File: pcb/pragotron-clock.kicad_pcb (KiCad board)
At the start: 2 copper layers, 60 x 60 mm, 11 parts, among them J1 Conn_01x02, J2 Conn_01x03, J3 Conn_01x03, J4 Conn_01x02, U1 L293D, U2 ESP32_DEVCITV1

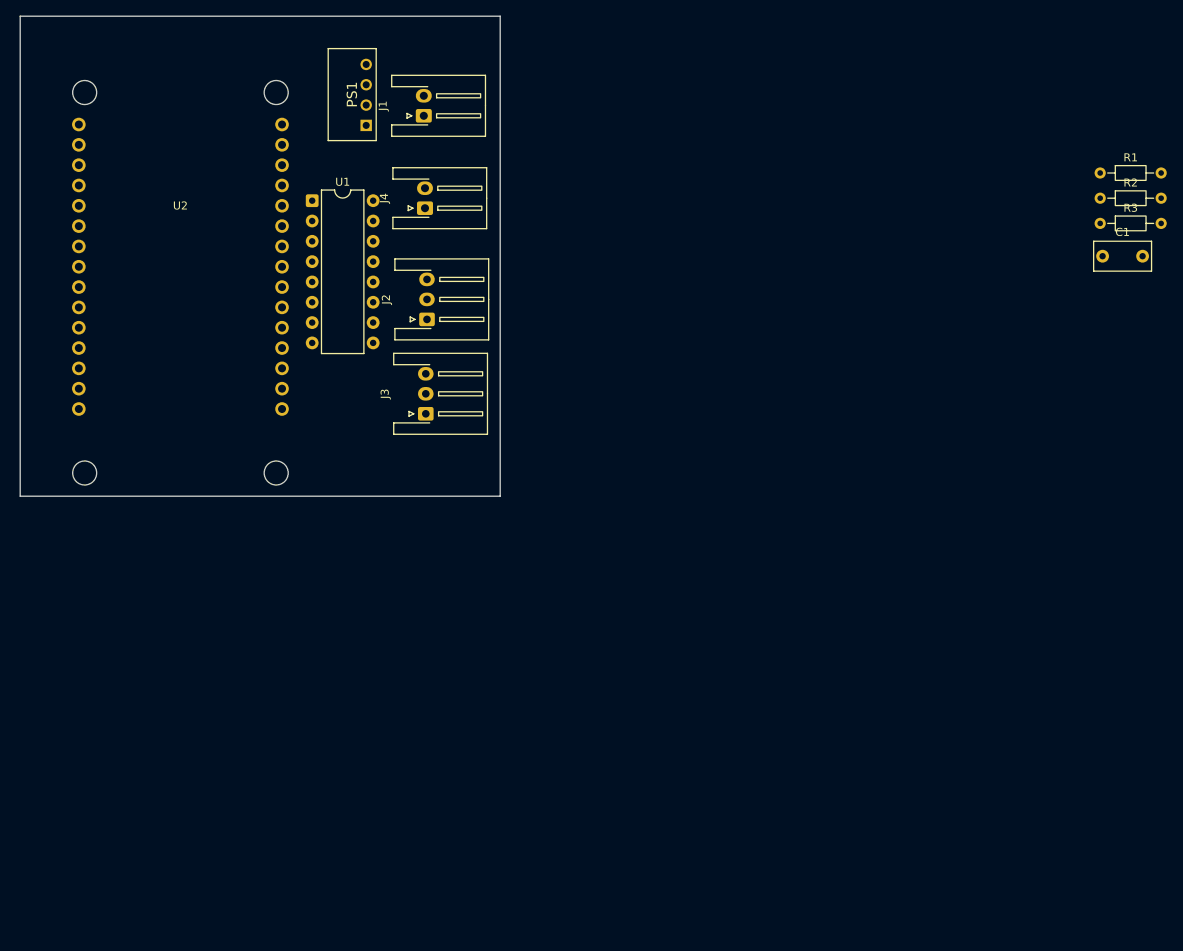
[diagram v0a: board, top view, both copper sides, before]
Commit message: schematic
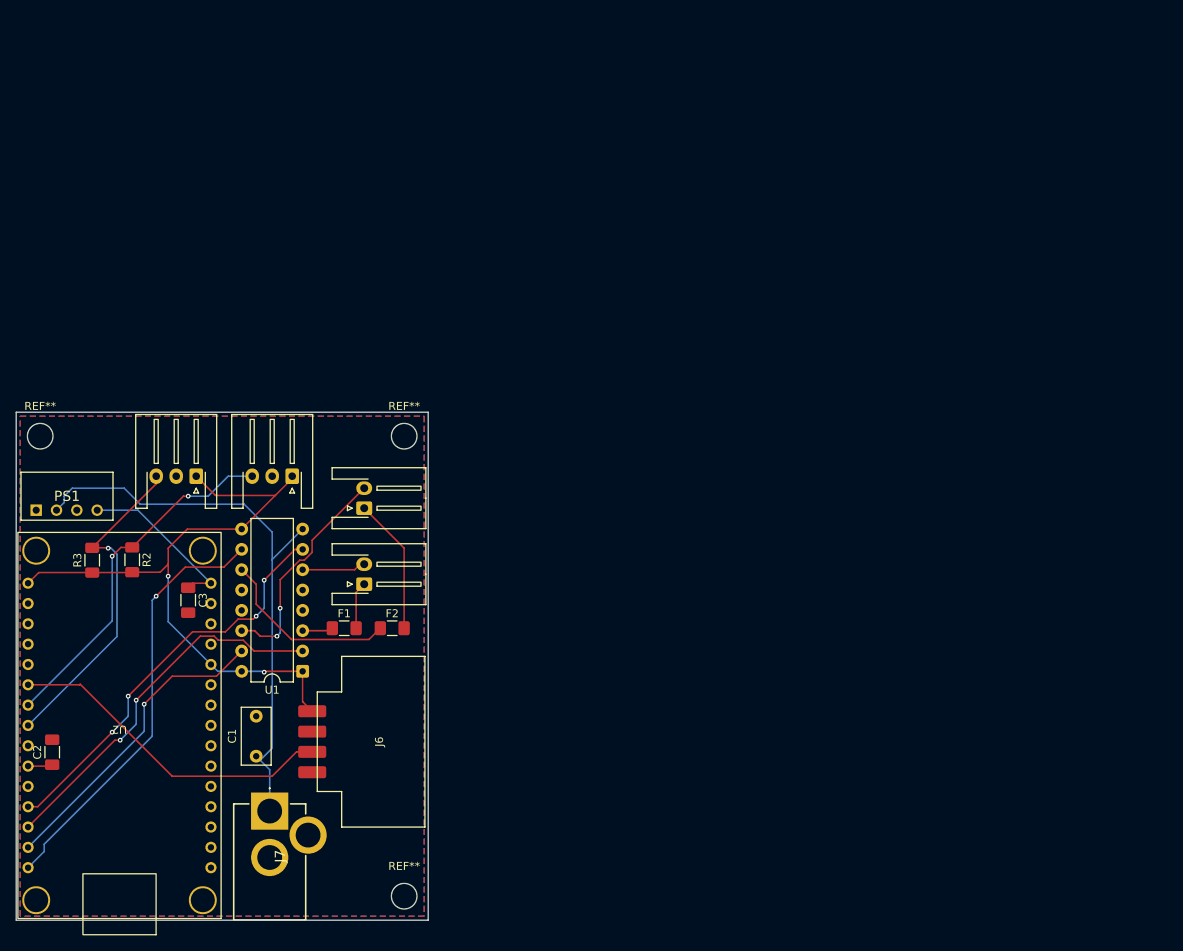
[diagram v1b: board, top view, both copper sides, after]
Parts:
- removed J4: Conn_01x02, Connector_JST:JST_XH_S2B-XH-A-1_1x02_P2.50mm_Horizontal
- removed R1: 47K, Resistor_THT:R_Axial_DIN0204_L3.6mm_D1.6mm_P7.62mm_Horizontal
- added C2: 100n, Capacitor_SMD:C_1206_3216Metric_Pad1.33x1.80mm_HandSolder, F.Cu at (84.0, 142.0)
- added C3: 100n, Capacitor_SMD:C_1206_3216Metric_Pad1.33x1.80mm_HandSolder, F.Cu at (101.0, 123.0)
- added F1: Fuse, Fuse:Fuse_1206_3216Metric_Pad1.42x1.75mm_HandSolder, F.Cu at (120.5, 126.5)
- added F2: Fuse, Fuse:Fuse_1206_3216Metric_Pad1.42x1.75mm_HandSolder, F.Cu at (126.5, 126.5)
- added J5: Conn_01x02, Connector_JST:JST_XH_S2B-XH-A-1_1x02_P2.50mm_Horizontal, F.Cu at (123.0, 111.5)
- added J6: Conn_01x04, JS_Local:DCF77, F.Cu at (125.4, 140.7)
- added J7: 694108301002, JS_Local:694108301002, F.Cu at (111.2, 149.4)
- added REF**: MountingHole_3.2mm_M3_DIN965, MountingHole:MountingHole_3.2mm_M3_DIN965, F.Cu at (128.0, 160.0)
- added REF**: MountingHole_3.2mm_M3_DIN965, MountingHole:MountingHole_3.2mm_M3_DIN965, F.Cu at (128.0, 102.5)
- added REF**: MountingHole_3.2mm_M3_DIN965, MountingHole:MountingHole_3.2mm_M3_DIN965, F.Cu at (82.5, 102.5)
- R2, R3: footprint Resistor_THT:R_Axial_DIN0204_L3.6mm_D1.6mm_P7.62mm_Horizontal -> Resistor_SMD:R_1206_3216Metric_Pad1.30x1.75mm_HandSolder
- U2: value ESP32_DEVCITV1 -> ~; footprint JS_Local:ESP32_DEVKITV1 -> JS_Local:ESP8266_12E_DEVKIT
- moved R3 132.8 mm to (89.0, 118.0), turned to 90 degrees
- moved R2 129.2 mm to (94.0, 118.0), turned to -90 degrees
- moved C1 122.9 mm to (109.5, 142.5), turned to 90 degrees
- moved U2 75.3 mm to (92.4, 138.7), turned to 180 degrees
- moved PS1 63.4 mm to (82.0, 111.8), turned to 0 degrees
- moved J1 59.0 mm to (123.0, 121.0)
- moved U1 58.8 mm to (115.3, 131.9), turned to 180 degrees
- moved J3 29.7 mm to (102.0, 107.5), turned to 180 degrees
- moved J2 25.8 mm to (114.0, 107.5), turned to 180 degrees
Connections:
- J2 pad 1: Net-(J2-Pin_1) -> +3V3
- J2 pad 3: Net-(J2-Pin_3) -> /SENS2
- J3 pad 1: Net-(J2-Pin_1) -> +3V3
- J3 pad 3: Net-(J3-Pin_3) -> /SENS1
- R2 pad 1: Net-(J2-Pin_3) -> /SENS2
- R2 pad 2: Net-(J2-Pin_1) -> +3V3
- R3 pad 1: Net-(J2-Pin_1) -> +3V3
- R3 pad 2: Net-(J3-Pin_3) -> /SENS1
- U1 pad 1: Net-(U1-EN1,2) -> +3V3
- U1 pad 10: unconnected-(U1-3A-Pad10) -> /OUT2_POSITIVE
- U1 pad 11: unconnected-(U1-3Y-Pad11) -> Net-(U1-3Y)
- U1 pad 14: unconnected-(U1-4Y-Pad14) -> Net-(J5-Pin_2)
- U1 pad 15: unconnected-(U1-4A-Pad15) -> /OUT2_NEGATIVE
- U1 pad 16: Net-(J2-Pin_1) -> +3V3
- U1 pad 2: Net-(U1-1A) -> /OUT1_POSITIVE
- U1 pad 3: Net-(J1-Pin_1) -> Net-(U1-1Y)
- U1 pad 7: Net-(U1-2A) -> /OUT1_NEGATIVE
- U1 pad 9: GND -> +3V3
- U2 pad 1: unconnected-(U2-EN-Pad1) -> /OUT2_POSITIVE
- U2 pad 10: unconnected-(U2-D27-Pad10) -> /DCF_SIG
- U2 pad 13: Net-(U1-EN1,2) -> unconnected-(U2-TX-Pad13)
- U2 pad 14: unconnected-(U2-GND-Pad14) -> GND
- U2 pad 15: +5V -> +3V3
- U2 pad 16: unconnected-(U2-D23-Pad16) -> +5V
- U2 pad 17: unconnected-(U2-D22-Pad17) -> GND
- U2 pad 2: unconnected-(U2-VP-Pad2) -> /OUT2_NEGATIVE
- U2 pad 20: unconnected-(U2-D21-Pad20) -> +3V3
- U2 pad 21: Net-(U1-1A) -> GND
- U2 pad 22: Net-(U1-2A) -> unconnected-(U2-CLK-Pad22)
- U2 pad 3: unconnected-(U2-VN-Pad3) -> /OUT1_POSITIVE
- U2 pad 30: Net-(J2-Pin_1) -> unconnected-(U2-A0-Pad30)
- U2 pad 4: unconnected-(U2-D34-Pad4) -> /OUT1_NEGATIVE
- U2 pad 5: Net-(J2-Pin_3) -> unconnected-(U2-D4-Pad5)
- U2 pad 6: Net-(J3-Pin_3) -> +3V3
- U2 pad 7: unconnected-(U2-D33-Pad7) -> GND
- U2 pad 8: unconnected-(U2-D25-Pad8) -> /SENS1
- U2 pad 9: unconnected-(U2-D26-Pad9) -> /SENS2
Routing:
- net +3V3: track 0.00 -> 86.0 mm, vias 0 -> 2
- net +24V: track 0.00 -> 73.0 mm
- net /OUT2_POSITIVE: track 0.00 -> 53.7 mm, vias 0 -> 1
- net /OUT1_NEGATIVE: track 0.00 -> 51.2 mm, vias 0 -> 4
- net /OUT1_POSITIVE: track 0.00 -> 46.7 mm, vias 0 -> 2
- net /SENS2: track 0.00 -> 44.6 mm, vias 0 -> 2
- net /SENS1: track 0.00 -> 41.7 mm, vias 0 -> 1
- net /DCF_SIG: track 0.00 -> 41.6 mm
- net /OUT2_NEGATIVE: track 0.00 -> 38.8 mm, vias 0 -> 1
- net Net-(J5-Pin_2): track 0.00 -> 28.1 mm, vias 0 -> 2
- net Net-(U1-3Y): track 0.00 -> 23.0 mm
- net +5V: track 0.00 -> 21.1 mm
- net Net-(J5-Pin_1): track 0.00 -> 17.1 mm
- net Net-(J1-Pin_2): track 0.00 -> 7.98 mm
- net Net-(J1-Pin_1): track 0.00 -> 5.92 mm
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- added copper zone on B.Cu, net GND
- added copper zone on F.Cu, net GND
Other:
- board size 60 x 60 mm -> 51.5 x 63.5 mm

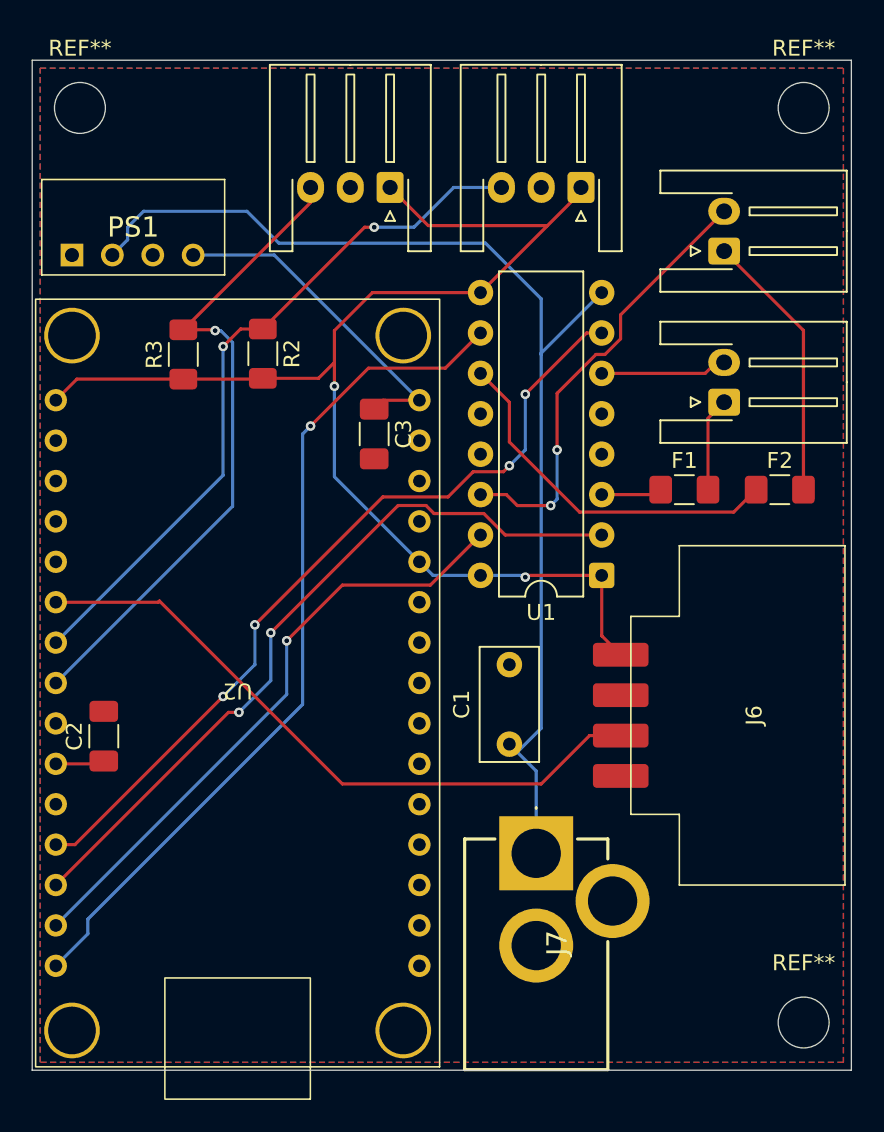
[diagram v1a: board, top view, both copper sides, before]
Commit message: minification
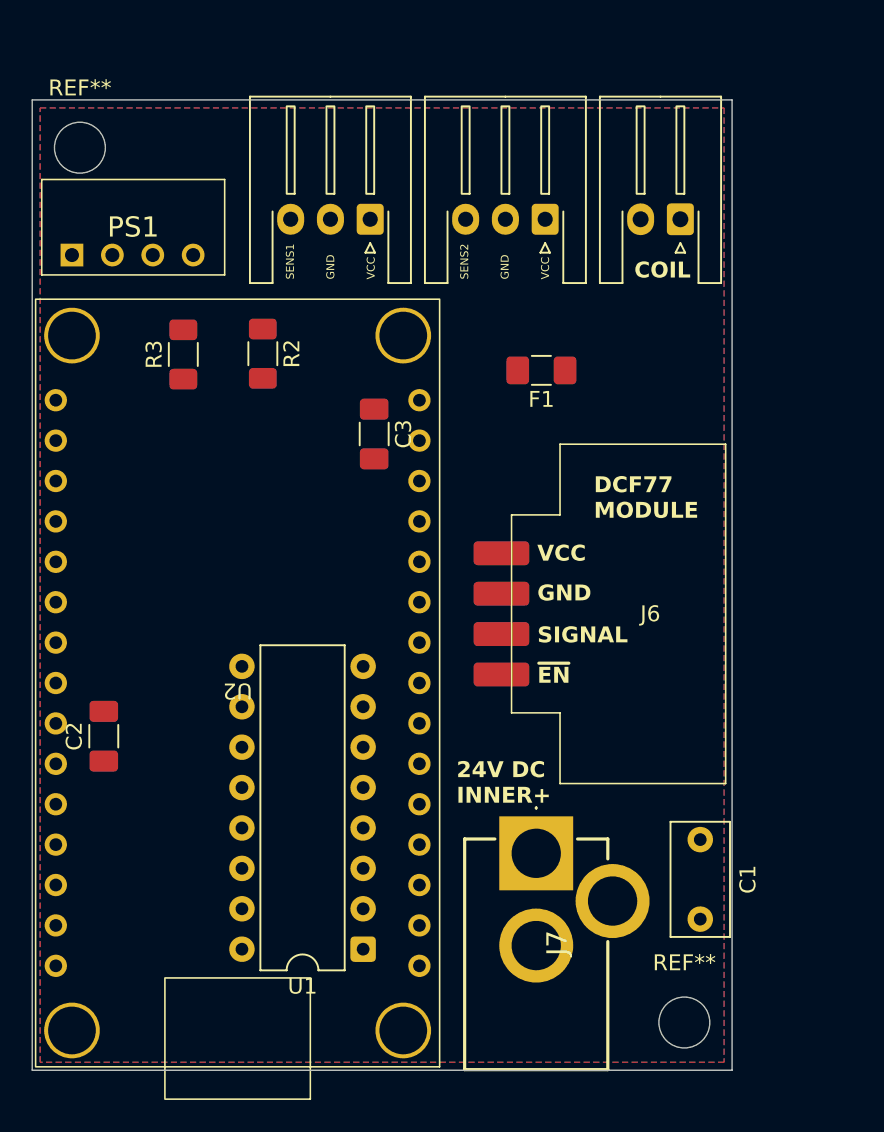
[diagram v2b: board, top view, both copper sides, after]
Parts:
- removed F2: Fuse, Fuse:Fuse_1206_3216Metric_Pad1.42x1.75mm_HandSolder
- removed J5: Conn_01x02, Connector_JST:JST_XH_S2B-XH-A-1_1x02_P2.50mm_Horizontal
- removed the REF** at (128.0, 102.5)
- moved U1 27.9 mm to (100.3, 155.4)
- moved C1 13.4 mm to (121.5, 148.5), turned to -90 degrees
- moved J1 11.8 mm to (120.2, 109.5), turned to 180 degrees
- moved F1 11.7 mm to (111.5, 119.0), turned to 180 degrees
- moved J6 9.85 mm to (117.9, 134.3)
- moved REF** 7.50 mm to (120.5, 160.0)
- moved J2 3.01 mm to (111.8, 109.5)
- moved REF** 2.50 mm to (82.5, 105.0)
- moved J3 2.36 mm to (100.8, 109.5)
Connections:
- U1 pad 10: /OUT2_POSITIVE -> unconnected-(U1-3A-Pad10)
- U1 pad 11: Net-(U1-3Y) -> unconnected-(U1-3Y-Pad11)
- U1 pad 14: Net-(J5-Pin_2) -> unconnected-(U1-4Y-Pad14)
- U1 pad 15: /OUT2_NEGATIVE -> unconnected-(U1-4A-Pad15)
- U1 pad 9: +3V3 -> GND
- U2 pad 1: /OUT2_POSITIVE -> unconnected-(U2-D0-Pad1)
- U2 pad 2: /OUT2_NEGATIVE -> unconnected-(U2-D1-Pad2)
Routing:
- net +3V3: track 86.0 -> 0.00 mm, vias 2 -> 0
- net +24V: track 73.0 -> 0.00 mm
- net /OUT2_POSITIVE: track 53.7 -> 0.00 mm, vias 1 -> 0
- net /OUT1_NEGATIVE: track 51.2 -> 0.00 mm, vias 4 -> 0
- net /OUT1_POSITIVE: track 46.7 -> 0.00 mm, vias 2 -> 0
- net /SENS2: track 44.6 -> 0.00 mm, vias 2 -> 0
- net /SENS1: track 41.7 -> 0.00 mm, vias 1 -> 0
- net /DCF_SIG: track 41.6 -> 0.00 mm
- net /OUT2_NEGATIVE: track 38.8 -> 0.00 mm, vias 1 -> 0
- net Net-(J5-Pin_2): track 28.1 -> 0.00 mm, vias 2 -> 0
- net Net-(U1-3Y): track 23.0 -> 0.00 mm
- net +5V: track 21.1 -> 0.00 mm
- net Net-(J5-Pin_1): track 17.1 -> 0.00 mm
- net Net-(J1-Pin_2): track 7.98 -> 0.00 mm
- net Net-(J1-Pin_1): track 5.92 -> 0.00 mm
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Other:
- board size 51.5 x 63.5 mm -> 44 x 61 mm
- board text added: "24V DC INNER+"
- board text added: "COIL"
- board text added: "DCF77 MODULE"
- board text added: "GND"
- board text added: "SENS1"
- board text added: "SENS2"
- board text added: "SIGNAL"
- board text added: "VCC"
- board text added: "~{EN}"
